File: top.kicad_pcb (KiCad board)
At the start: 2 copper layers, 96.5 x 46 mm, 4 parts, among them J2 Conn_01x01_Male, J5 Conn_01x01_Male, J7 Conn_01x01_Male, J9 Conn_01x01_Male

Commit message: gerberek, bom
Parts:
- added T1: Tab, kikit:Tab, F.Cu at (82.2, 68.0)
- added T1: Tab, kikit:Tab, F.Cu at (164.8, 57.6)
- added T1: Tab, kikit:Tab, F.Cu at (82.2, 94.0)
- added T1: Tab, kikit:Tab, F.Cu at (179.8, 94.0)
- added T1: Tab, kikit:Tab, F.Cu at (95.8, 57.6)
- added T1: Tab, kikit:Tab, F.Cu at (95.8, 104.3)
- added T1: Tab, kikit:Tab, F.Cu at (164.8, 104.3)
- added T1: Tab, kikit:Tab, F.Cu at (179.6, 68.4)
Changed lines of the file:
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@@
     )
+  )
+  (footprint "kikit:Tab" (layer "F.Cu")
+    (at 82.25 68)
+    (descr "A symbol representing annotation for tab placement")
+    (property "Sheetfile" "SEM15.kicad_sch")
+    (property "Sheetname" "")
+    (property "exclude_from_bom" "")
+    (property "ki_description" "KiKit tab annotations")
+    (property "ki_keywords" "KiKit")
+    (attr exclude_from_pos_files exclude_from_bom)
+    (fp_text reference "T1" (at 0 -2) (layer "F.SilkS") hide
+        (effects (font (size 1 1) (thickness 0.15)))
+    )
+    (fp_text value "Tab" (at -2.75 -1) (layer "Dwgs.User")
+        (effects (font (size 1.2 1.2) (thickness 0.2)))
+    )
+    (fp_text user "KIKIT: width: 3mm" (at -5.5 0 90) (layer "Dwgs.User")
+        (effects (font (size 1 1) (thickness 0.15)))
+    )
+    (fp_line (start 0.25 0) (end -2.75 0)
+      (stroke (width 0.3) (type solid)) (layer "Dwgs.User"))
+    (fp_line (start 0.25 0) (end -0.75 -1)
+      (stroke (width 0.3) (type solid)) (layer "Dwgs.User"))
+    (fp_line (start 0.25 0) (end -0.75 1)
+      (stroke (width 0.3) (type solid)) (layer "Dwgs.User"))
+    (fp_line (start 0.25 1) (end 0.25 -1)
+      (stroke (width 0.3) (type solid)) (layer "Dwgs.User"))
+  )
+  (footprint "kikit:Tab" (layer "F.Cu")
+    (at 164.8 57.65 -90)
+    (descr "A symbol representing annotation for tab placement")
+    (property "Sheetfile" "SEM15.kicad_sch")
+    (property "Sheetname" "")
+    (property "exclude_from_bom" "")
+    (property "ki_description" "KiKit tab annotations")
+    (property "ki_keywords" "KiKit")
+    (attr exclude_from_pos_files exclude_from_bom)
+    (fp_text reference "T1" (at 0 -2 90) (layer "F.SilkS") hide
+        (effects (font (size 1 1) (thickness 0.15)))
+    )
+    (fp_text value "Tab" (at -2.75 -1 90) (layer "Dwgs.User")
+        (effects (font (size 1.2 1.2) (thickness 0.2)))
+    )
+    (fp_text user "KIKIT: width: 3mm" (at -5.5 0) (layer "Dwgs.User")
+        (effects (font (size 1 1) (thickness 0.15)))
+    )
+    (fp_line (start 0.25 0) (end -2.75 0)
+      (stroke (width 0.3) (type solid)) (layer "Dwgs.User"))
+    (fp_line (start 0.25 0) (end -0.75 -1)
+      (stroke (width 0.3) (type solid)) (layer "Dwgs.User"))
+    (fp_line (start 0.25 0) (end -0.75 1)
+      (stroke (width 0.3) (type solid)) (layer "Dwgs.User"))
+    (fp_line (start 0.25 1) (end 0.25 -1)
+      (stroke (width 0.3) (type solid)) (layer "Dwgs.User"))
+  )
+  (footprint "kikit:Tab" (layer "F.Cu")
+    (at 82.25 94)
+    (descr "A symbol representing annotation for tab placement")
+    (property "Sheetfile" "SEM15.kicad_sch")
+    (property "Sheetname" "")
+    (property "exclude_from_bom" "")
+    (property "ki_description" "KiKit tab annotations")
+    (property "ki_keywords" "KiKit")
+    (attr exclude_from_pos_files exclude_from_bom)
+    (fp_text reference "T1" (at 0 -2) (layer "F.SilkS") hide
+        (effects (font (size 1 1) (thickness 0.15)))
+    )
+    (fp_text value "Tab" (at -2.75 -1) (layer "Dwgs.User")
+        (effects (font (size 1.2 1.2) (thickness 0.2)))
+    )
+    (fp_text user "KIKIT: width: 3mm" (at -5.5 0 90) (layer "Dwgs.User")
+        (effects (font (size 1 1) (thickness 0.15)))
+    )
+    (fp_line (start 0.25 0) (end -2.75 0)
+      (stroke (width 0.3) (type solid)) (layer "Dwgs.User"))
+    (fp_line (start 0.25 0) (end -0.75 -1)
+      (stroke (width 0.3) (type solid)) (layer "Dwgs.User"))
+    (fp_line (start 0.25 0) (end -0.75 1)
+      (stroke (width 0.3) (type solid)) (layer "Dwgs.User"))
+    (fp_line (start 0.25 1) (end 0.25 -1)
+      (stroke (width 0.3) (type solid)) (layer "Dwgs.User"))
+  )
+  (footprint "kikit:Tab" (layer "F.Cu")
+    (at 179.75 94 180)
+    (descr "A symbol representing annotation for tab placement")
+    (property "Sheetfile" "SEM15.kicad_sch")
+    (property "Sheetname" "")
+    (property "exclude_from_bom" "")
+    (property "ki_description" "KiKit tab annotations")
+    (property "ki_keywords" "KiKit")
+    (attr exclude_from_pos_files exclude_from_bom)
+    (fp_text reference "T1" (at 0 -2) (layer "F.SilkS") hide
+        (effects (font (size 1 1) (thickness 0.15)))
+    )
+    (fp_text value "Tab" (at -2.75 -1) (layer "Dwgs.User")
+        (effects (font (size 1.2 1.2) (thickness 0.2)))
+    )
+    (fp_text user "KIKIT: width: 3mm" (at -5.5 0 90) (layer "Dwgs.User")
+        (effects (font (size 1 1) (thickness 0.15)))
+    )
+    (fp_line (start 0.25 0) (end -2.75 0)
+      (stroke (width 0.3) (type solid)) (layer "Dwgs.User"))
+    (fp_line (start 0.25 0) (end -0.75 -1)
+      (stroke (width 0.3) (type solid)) (layer "Dwgs.User"))
+    (fp_line (start 0.25 0) (end -0.75 1)
+      (stroke (width 0.3) (type solid)) (layer "Dwgs.User"))
+    (fp_line (start 0.25 1) (end 0.25 -1)
+      (stroke (width 0.3) (type solid)) (layer "Dwgs.User"))
   )
   (footprint "Connector_PinHeader_2.54mm:PinHeader_1x01_P2.54mm_Vertical" (layer "F.Cu")
@@
     )
   )
+  (footprint "kikit:Tab" (layer "F.Cu")
+    (at 95.8 57.65 -90)
+    (descr "A symbol representing annotation for tab placement")
+    (property "Sheetfile" "SEM15.kicad_sch")
+    (property "Sheetname" "")
+    (property "exclude_from_bom" "")
+    (property "ki_description" "KiKit tab annotations")
+    (property "ki_keywords" "KiKit")
+    (attr exclude_from_pos_files exclude_from_bom)
+    (fp_text reference "T1" (at 0 -2 90) (layer "F.SilkS") hide
+        (effects (font (size 1 1) (thickness 0.15)))
+    )
+    (fp_text value "Tab" (at -2.75 -1 90) (layer "Dwgs.User")
+        (effects (font (size 1.2 1.2) (thickness 0.2)))
+    )
+    (fp_text user "KIKIT: width: 3mm" (at -5.5 0) (layer "Dwgs.User")
+        (effects (font (size 1 1) (thickness 0.15)))
+    )
+    (fp_line (start 0.25 0) (end -2.75 0)
+      (stroke (width 0.3) (type solid)) (layer "Dwgs.User"))
+    (fp_line (start 0.25 0) (end -0.75 -1)
+      (stroke (width 0.3) (type solid)) (layer "Dwgs.User"))
+    (fp_line (start 0.25 0) (end -0.75 1)
+      (stroke (width 0.3) (type solid)) (layer "Dwgs.User"))
+    (fp_line (start 0.25 1) (end 0.25 -1)
+      (stroke (width 0.3) (type solid)) (layer "Dwgs.User"))
+  )
   (footprint "Connector_PinHeader_2.54mm:PinHeader_1x01_P2.54mm_Vertical" (layer "F.Cu")
     (at 95.7 102)
@@
     )
   )
+  (footprint "kikit:Tab" (layer "F.Cu")
+    (at 95.8 104.35 90)
+    (descr "A symbol representing annotation for tab placement")
+    (property "Sheetfile" "SEM15.kicad_sch")
+    (property "Sheetname" "")
+    (property "exclude_from_bom" "")
+    (property "ki_description" "KiKit tab annotations")
+    (property "ki_keywords" "KiKit")
+    (attr exclude_from_pos_files exclude_from_bom)
+    (fp_text reference "T1" (at 0 -2 90) (layer "F.SilkS") hide
+        (effects (font (size 1 1) (thickness 0.15)))
+    )
+    (fp_text value "Tab" (at -2.75 -1 90) (layer "Dwgs.User")
+        (effects (font (size 1.2 1.2) (thickness 0.2)))
+    )
+    (fp_text user "KIKIT: width: 3mm" (at -5.5 0) (layer "Dwgs.User")
+        (effects (font (size 1 1) (thickness 0.15)))
+    )
+    (fp_line (start 0.25 0) (end -2.75 0)
+      (stroke (width 0.3) (type solid)) (layer "Dwgs.User"))
+    (fp_line (start 0.25 0) (end -0.75 -1)
+      (stroke (width 0.3) (type solid)) (layer "Dwgs.User"))
+    (fp_line (start 0.25 0) (end -0.75 1)
+      (stroke (width 0.3) (type solid)) (layer "Dwgs.User"))
+    (fp_line (start 0.25 1) (end 0.25 -1)
+      (stroke (width 0.3) (type solid)) (layer "Dwgs.User"))
+  )
+  (footprint "kikit:Tab" (layer "F.Cu")
+    (at 164.8 104.35 90)
+    (descr "A symbol representing annotation for tab placement")
+    (property "Sheetfile" "SEM15.kicad_sch")
+    (property "Sheetname" "")
+    (property "exclude_from_bom" "")
+    (property "ki_description" "KiKit tab annotations")
+    (property "ki_keywords" "KiKit")
+    (attr exclude_from_pos_files exclude_from_bom)
+    (fp_text reference "T1" (at 0 -2 90) (layer "F.SilkS") hide
+        (effects (font (size 1 1) (thickness 0.15)))
+    )
+    (fp_text value "Tab" (at -2.75 -1 90) (layer "Dwgs.User")
+        (effects (font (size 1.2 1.2) (thickness 0.2)))
+    )
+    (fp_text user "KIKIT: width: 3mm" (at -5.5 0) (layer "Dwgs.User")
+        (effects (font (size 1 1) (thickness 0.15)))
+    )
+    (fp_line (start 0.25 0) (end -2.75 0)
+      (stroke (width 0.3) (type solid)) (layer "Dwgs.User"))
+    (fp_line (start 0.25 0) (end -0.75 -1)
+      (stroke (width 0.3) (type solid)) (layer "Dwgs.User"))
+    (fp_line (start 0.25 0) (end -0.75 1)
+      (stroke (width 0.3) (type solid)) (layer "Dwgs.User"))
+    (fp_line (start 0.25 1) (end 0.25 -1)
+      (stroke (width 0.3) (type solid)) (layer "Dwgs.User"))
+  )
+  (footprint "kikit:Tab" (layer "F.Cu")
+    (at 179.55 68.4 180)
+    (descr "A symbol representing annotation for tab placement")
+    (property "Sheetfile" "SEM15.kicad_sch")
+    (property "Sheetname" "")
+    (property "exclude_from_bom" "")
+    (property "ki_description" "KiKit tab annotations")
+    (property "ki_keywords" "KiKit")
+    (attr exclude_from_pos_files exclude_from_bom)
+    (fp_text reference "T1" (at 0 -2) (layer "F.SilkS") hide
+        (effects (font (size 1 1) (thickness 0.15)))
+    )
+    (fp_text value "Tab" (at -2.75 -1) (layer "Dwgs.User")
+        (effects (font (size 1.2 1.2) (thickness 0.2)))
+    )
+    (fp_text user "KIKIT: width: 3mm" (at -5.5 0 90) (layer "Dwgs.User")
+        (effects (font (size 1 1) (thickness 0.15)))
+    )
+    (fp_line (start 0.25 0) (end -2.75 0)
+      (stroke (width 0.3) (type solid)) (layer "Dwgs.User"))
+    (fp_line (start 0.25 0) (end -0.75 -1)
+      (stroke (width 0.3) (type solid)) (layer "Dwgs.User"))
+    (fp_line (start 0.25 0) (end -0.75 1)
+      (stroke (width 0.3) (type solid)) (layer "Dwgs.User"))
+    (fp_line (start 0.25 1) (end 0.25 -1)
+      (stroke (width 0.3) (type solid)) (layer "Dwgs.User"))
+  )
   (gr_line (start 156.214214 92.014214) (end 156.214214 66.014214)

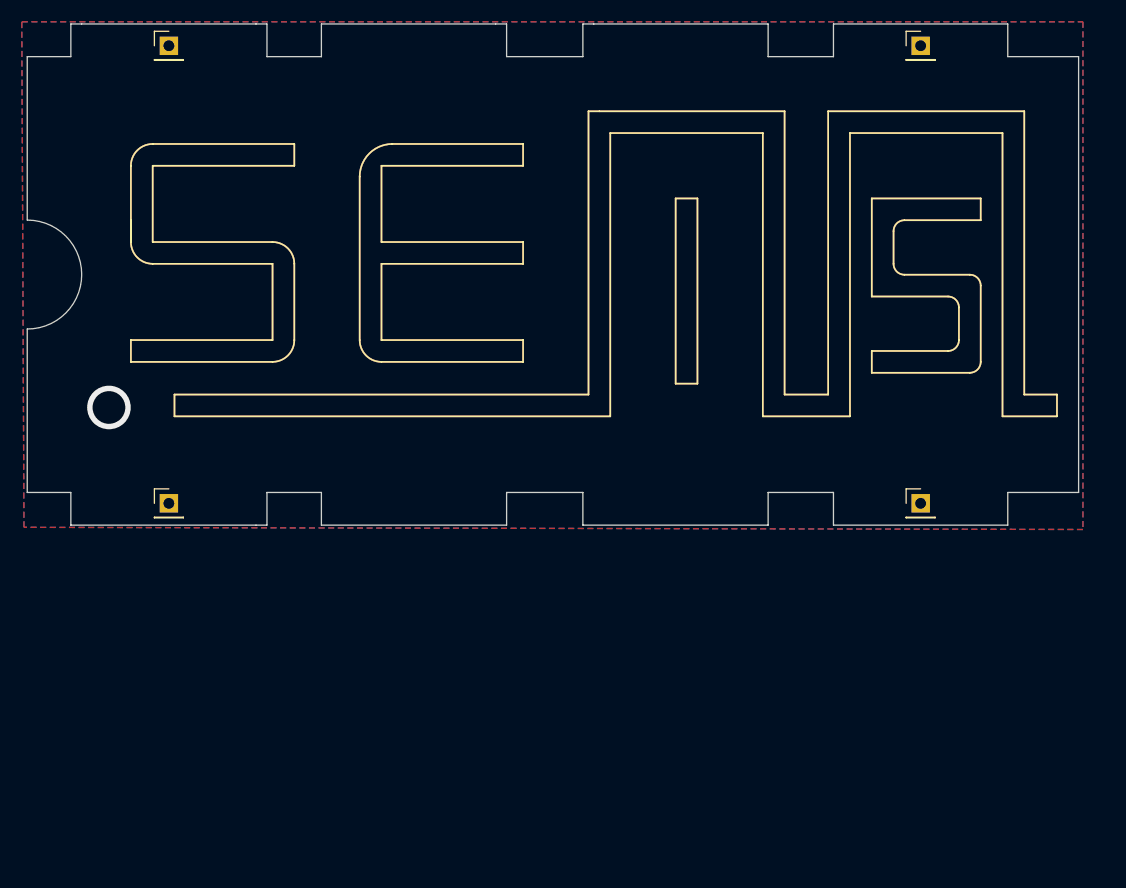
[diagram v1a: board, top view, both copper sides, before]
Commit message: sent to jlc
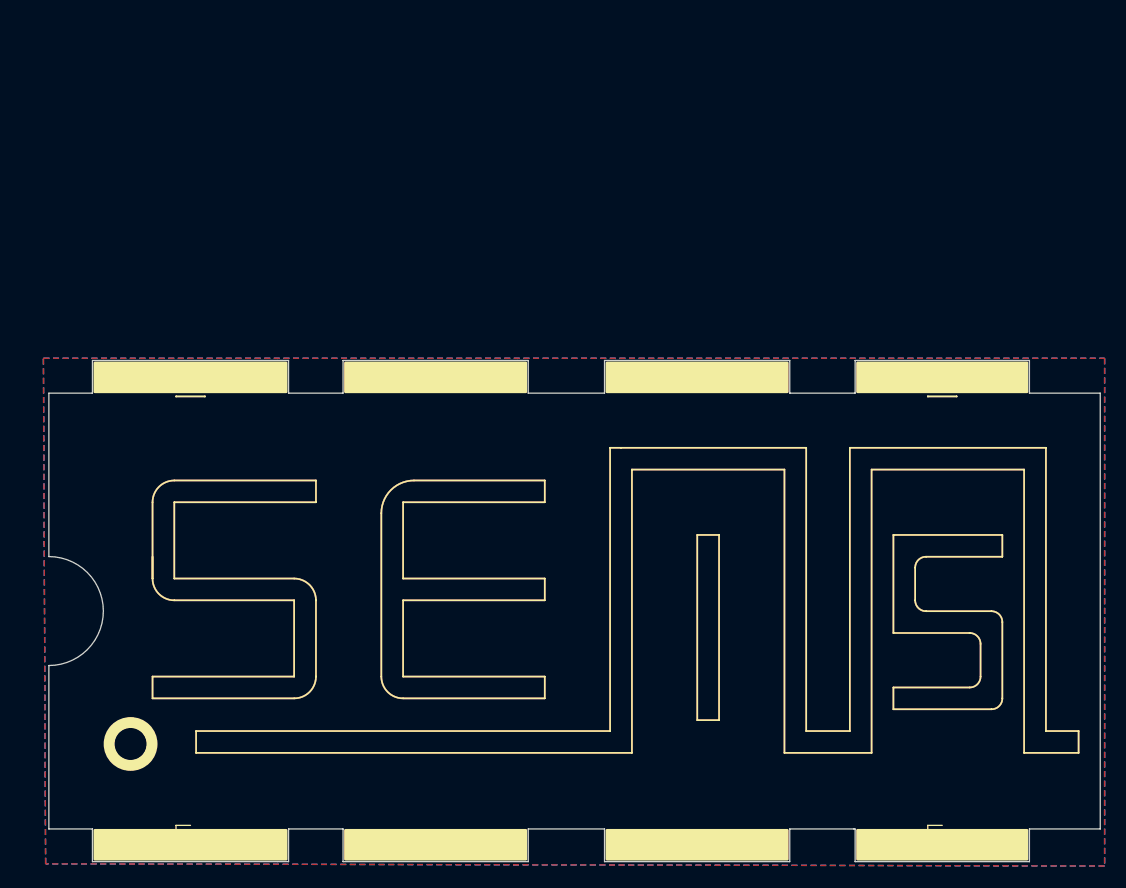
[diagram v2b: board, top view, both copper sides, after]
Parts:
- removed the T1 at (82.2, 68.0)
- removed the T1 at (164.8, 57.6)
- removed the T1 at (82.2, 94.0)
- removed the T1 at (179.8, 94.0)
- removed the T1 at (95.8, 57.6)
- removed the T1 at (95.8, 104.3)
- removed the T1 at (164.8, 104.3)
- removed the T1 at (179.6, 68.4)
- added T1: Tab, kikit:Tab, F.Cu at (84.2, 98.9)
- added T1: Tab, kikit:Tab, F.Cu at (181.5, 99.3)
- added T1: Tab, kikit:Tab, F.Cu at (181.7, 124.9)
- added T1: Tab, kikit:Tab, F.Cu at (166.8, 88.5)
- added T1: Tab, kikit:Tab, F.Cu at (97.8, 135.2)
- added T1: Tab, kikit:Tab, F.Cu at (84.2, 124.9)
- added T1: Tab, kikit:Tab, F.Cu at (97.8, 88.5)
- added T1: Tab, kikit:Tab, F.Cu at (166.8, 135.2)
- moved J2 30.9 mm to (97.7, 132.9)
- moved J5 30.9 mm to (166.7, 132.9)
- moved J7 30.9 mm to (166.7, 90.9)
- moved J9 30.9 mm to (97.7, 90.9)
